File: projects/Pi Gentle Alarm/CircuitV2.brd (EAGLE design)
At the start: 85.1 x 57.2 mm, 5 parts, among them X1 RASPI_BOARD_B+_E4, X2 22-23-2021

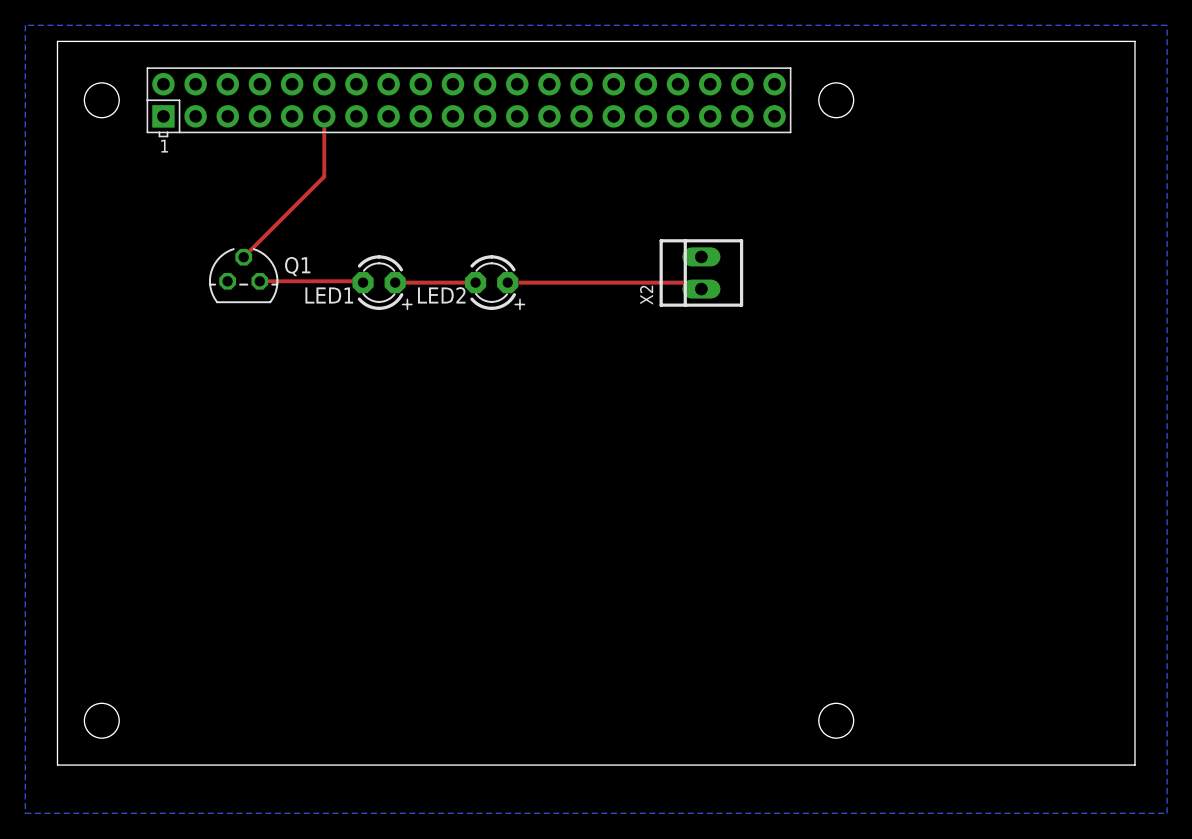
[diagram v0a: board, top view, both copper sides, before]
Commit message: Added template to board
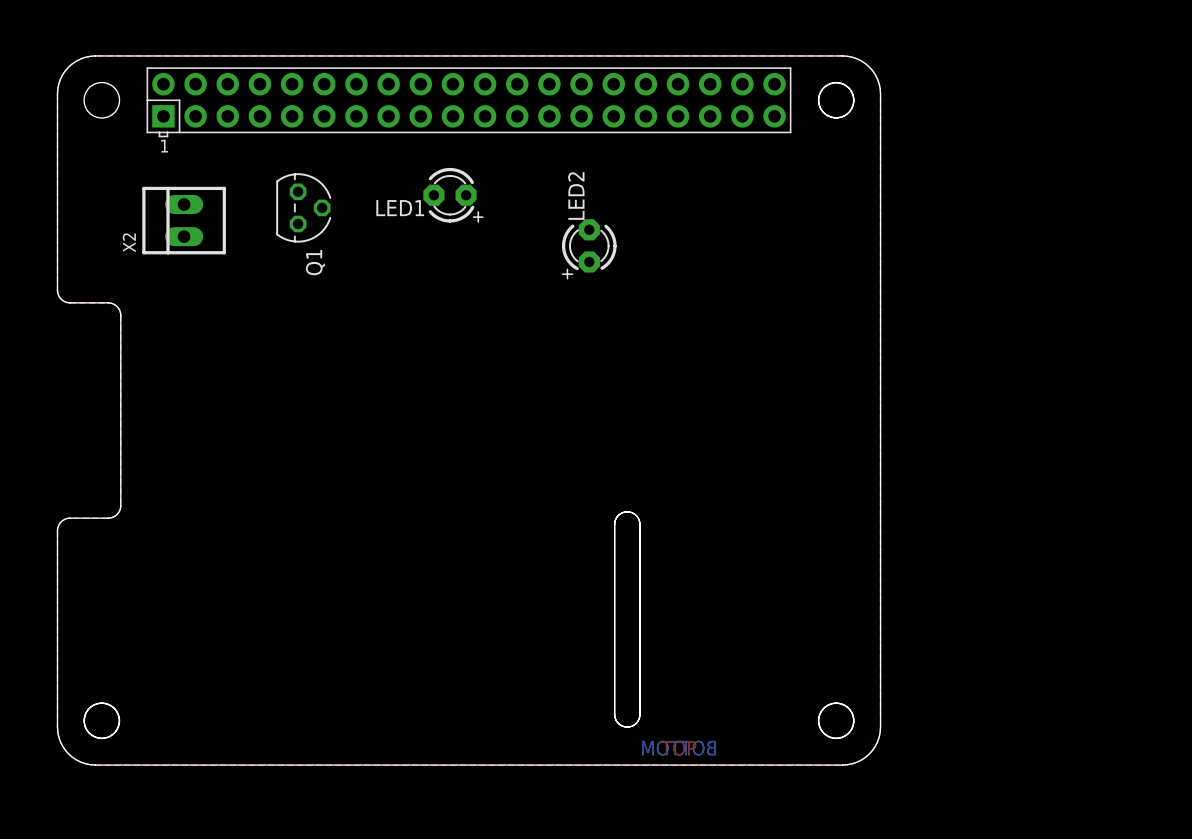
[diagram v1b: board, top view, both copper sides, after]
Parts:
- X1: value RASPI_BOARD_B+_E4 -> RASPI_BOARD_B+_E3; device raspberrypi_bastelstube_v13:RASPI_BOARD_B+_EDGES_4DRILL -> raspberrypi_bastelstube_v13:RASPI_BOARD_B+_EDGES_3DRILL
- moved X2 41.1 mm to (10.0, 43.0)
- moved LED1 8.89 mm to (31.0, 45.0)
- moved LED2 8.24 mm to (42.0, 41.0), turned to 90 degrees
- moved Q1 7.21 mm to (19.0, 44.0), turned to 270 degrees
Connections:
- net 5V0 renamed N$2
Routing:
- net VCC: track 15.5 -> 0.00 mm
- net GPIO17: track 13.8 -> 0.00 mm
- net N$6: track 8.20 -> 0.00 mm
- net N$1: track 6.35 -> 0.00 mm
- added copper zone on layer 1, net GND
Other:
- board size 85.1 x 57.2 mm -> 65 x 56 mm
- board text added: "BOTTOM"
- board text added: "TOP"
